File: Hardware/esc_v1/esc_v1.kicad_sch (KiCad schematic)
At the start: 27 parts, among them J1 vcc_connector, J2 SWD_tag_connect, J3 motor_connector, J4 10118193-0001LF

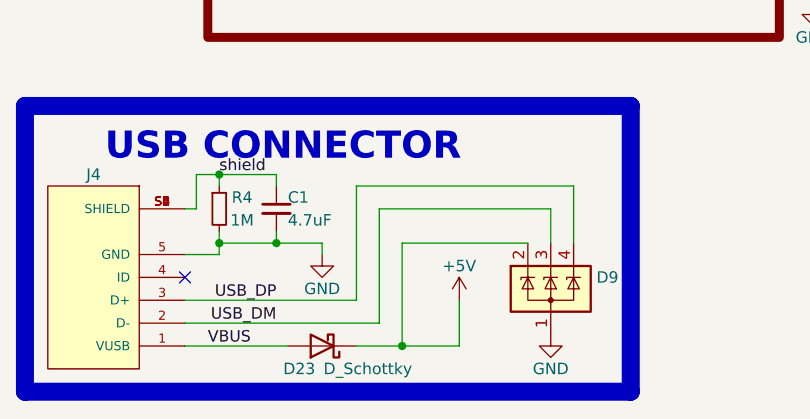
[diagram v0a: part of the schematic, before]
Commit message: Continued on layout
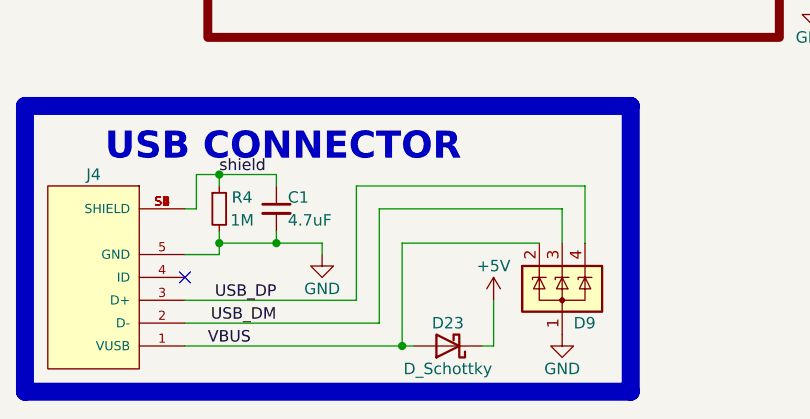
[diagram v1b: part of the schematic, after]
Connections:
- net +5V: no longer D9.2 (K)
- net VBUS: now also D9.2 (K)
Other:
- moved on the sheet: D23, D9
